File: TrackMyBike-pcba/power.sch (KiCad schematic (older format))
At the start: 43 parts

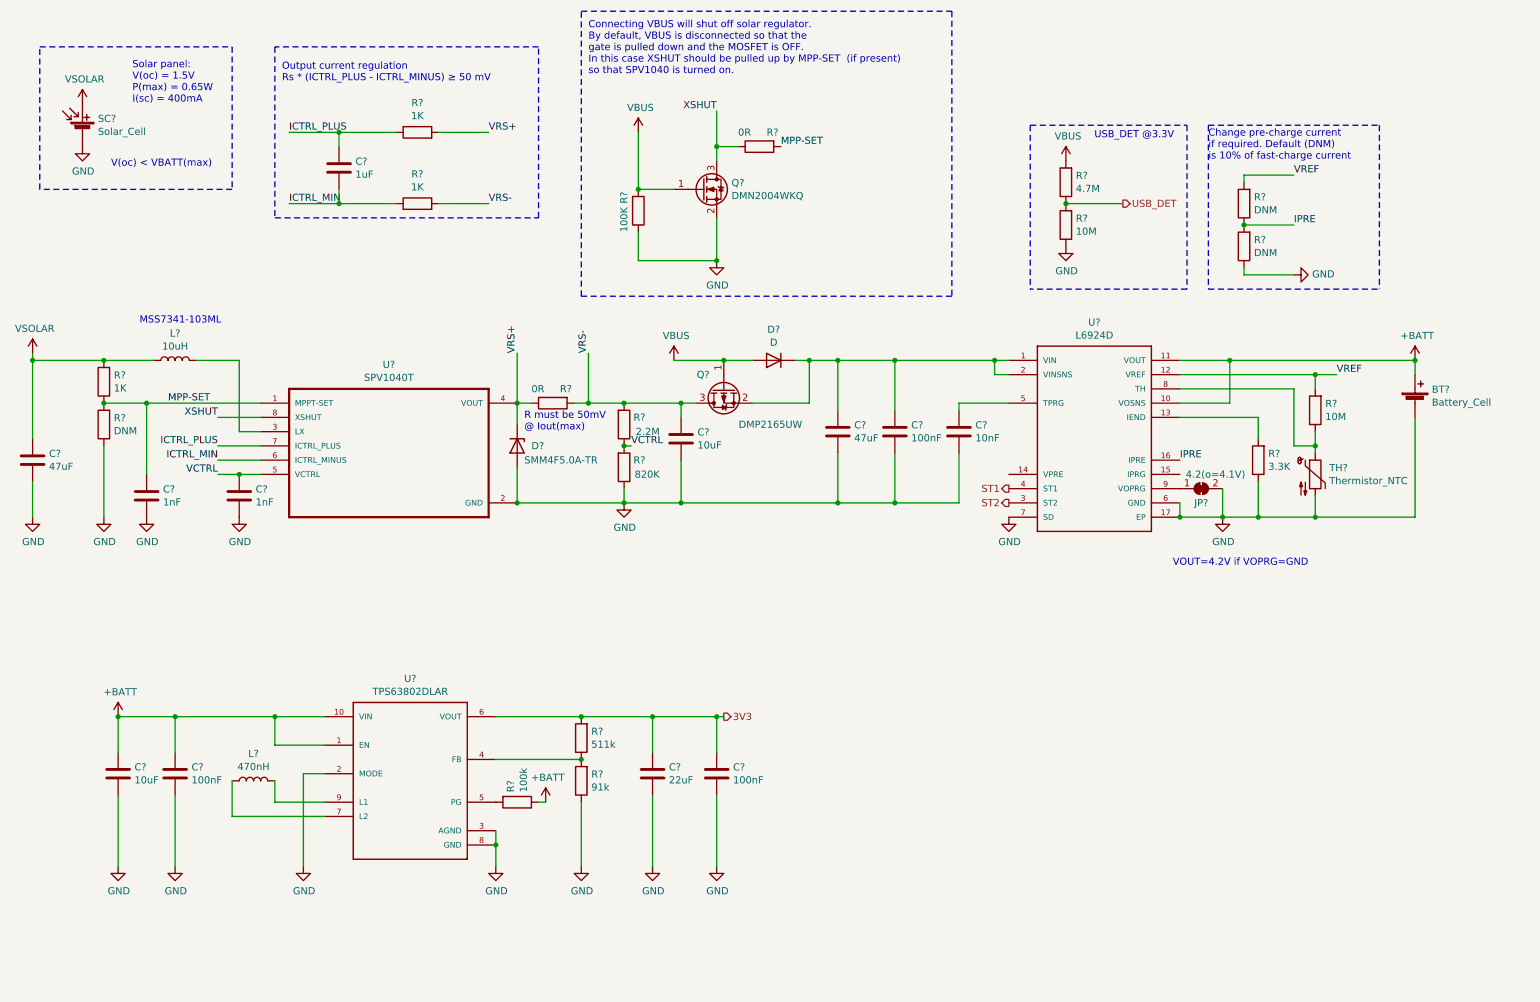
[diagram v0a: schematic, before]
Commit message: Modify power.sch
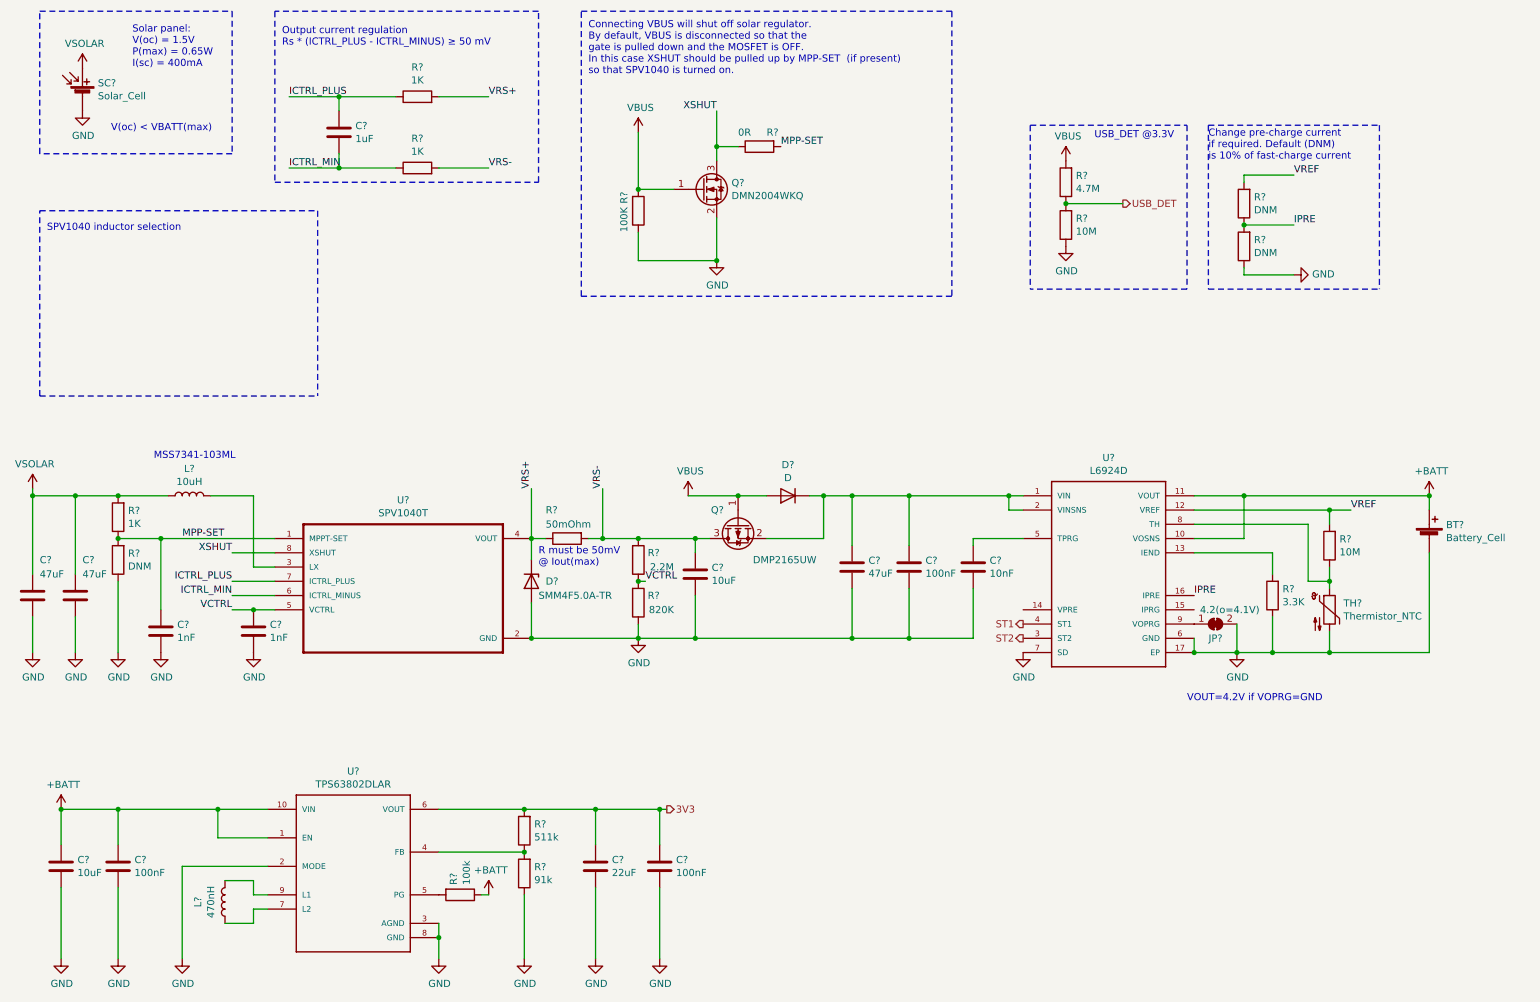
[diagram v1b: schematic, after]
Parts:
- added C?: 47uF, symbol Device:C
- R?: value 0R -> 50mOhm
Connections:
- net +1V0: now also C?.1
- net GND: now also C?.2
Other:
- note added: "SPV1040 inductor selection"
- moved on the sheet: BT?, C?, D?, JP?, L?, Q?, R?, SC?, TH?, U?
